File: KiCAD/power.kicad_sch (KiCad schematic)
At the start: 64 parts, among them IC10 ADP7182ACPZN-R7, IC11 NCP161ASN330T1G, IC4 NCP161ASN330T1G, IC5 NCP161ASN330T1G, IC6 NCP161ASN330T1G, IC7 NCP161ASN330T1G, IC8 LT1026CS8#PBF, IC9 ADP7118ARDZ

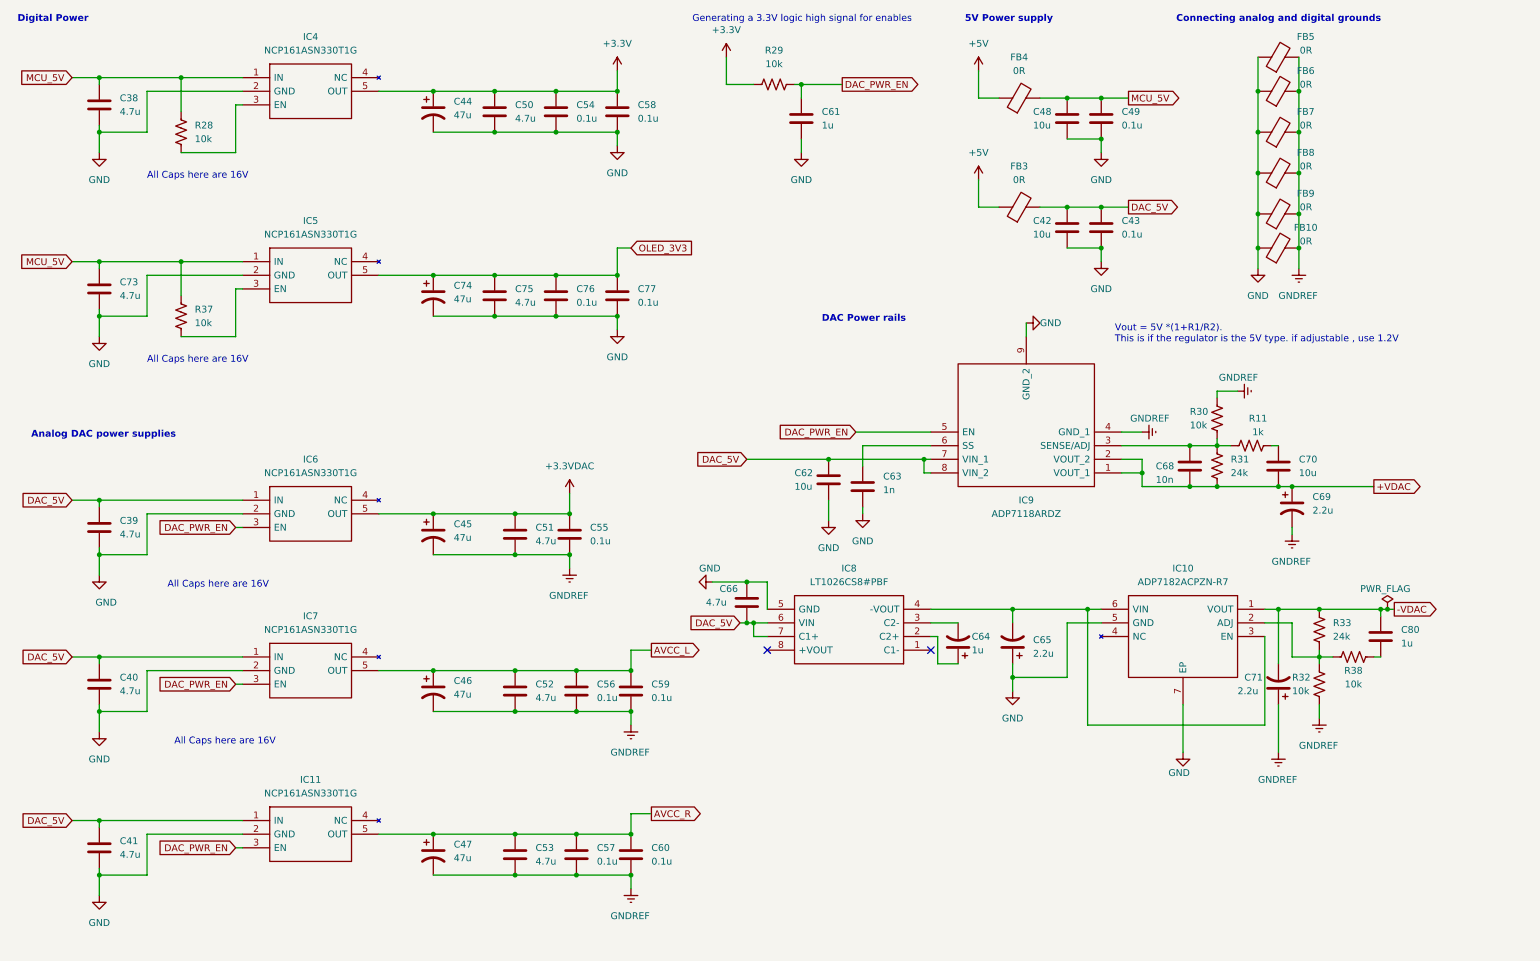
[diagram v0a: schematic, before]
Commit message: Adding stuff for rev 2.0
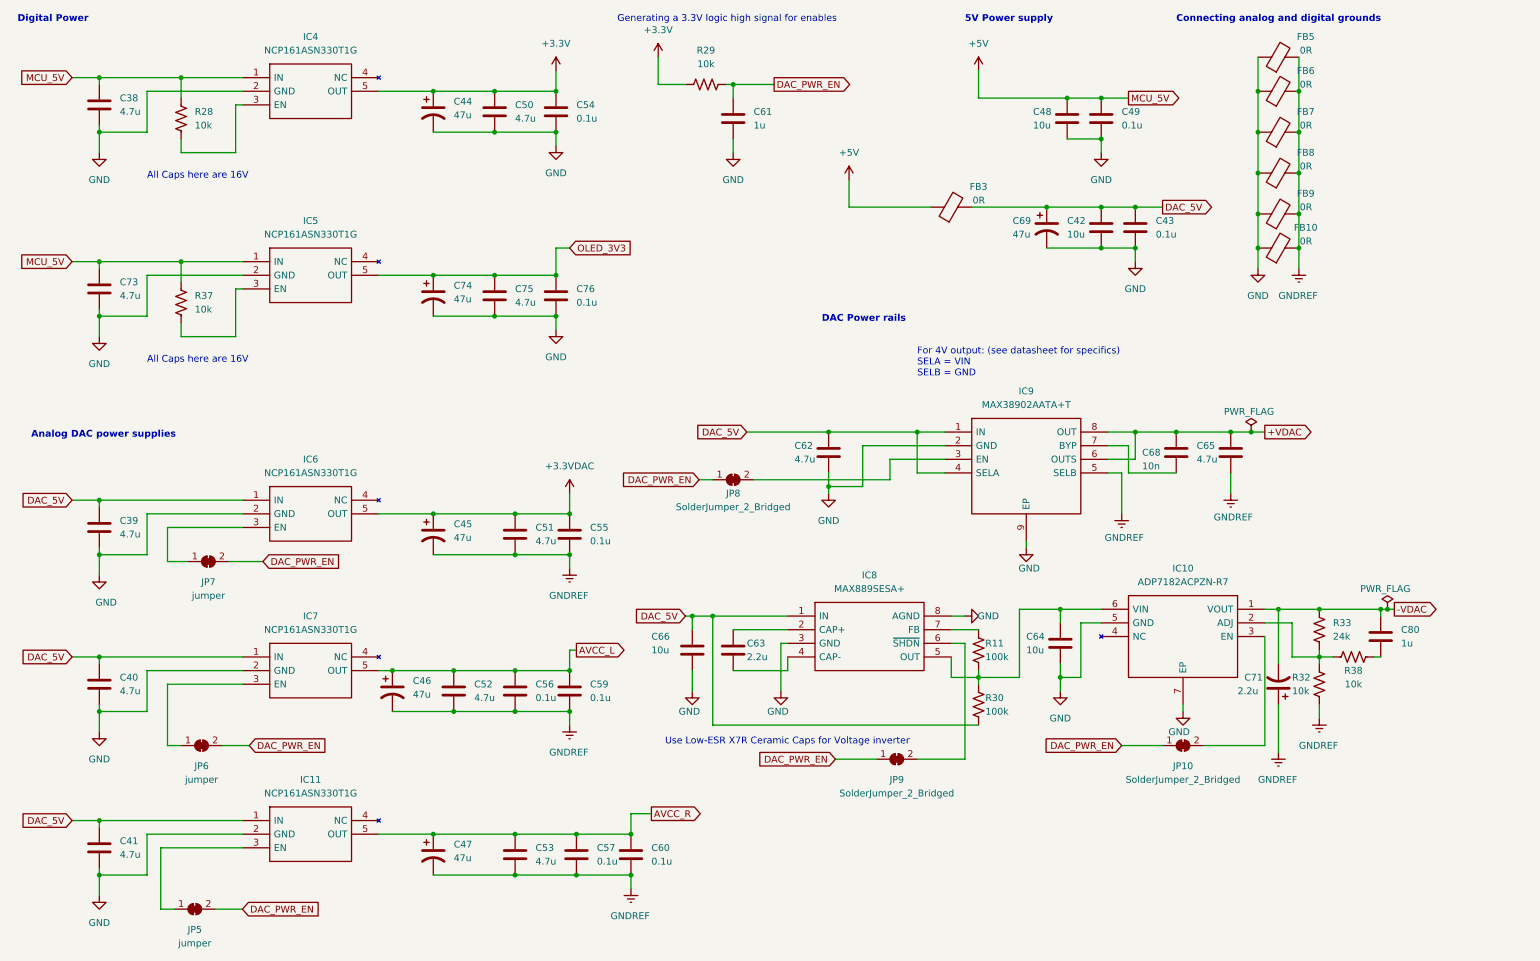
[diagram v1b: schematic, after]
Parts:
- removed C58, C77: 0.1u, Capacitor_SMD:C_0805_2012Metric_Pad1.18x1.45mm_HandSolder, symbol Device:C
- removed C64: 1u, Capacitor_THT:CP_Radial_D5.0mm_P2.00mm, symbol Device:C_Polarized_US
- removed C65: 2.2u, Capacitor_THT:CP_Radial_D4.0mm_P1.50mm, symbol Device:C_Polarized_US
- removed C70: 10u, Capacitor_SMD:C_0805_2012Metric_Pad1.18x1.45mm_HandSolder, symbol Device:C
- removed FB4: 0R, SamacSys_Parts:BEADC2012X110N, symbol Device:FerriteBead
- removed IC8: LT1026CS8#PBF, SamacSys_Parts:SOIC127P599X175-8N, symbol SamacSys_Parts:LT1026CS8#PBF
- removed IC9: ADP7118ARDZ, SOIC127P600X175-9N, symbol SamacSys_Parts:ADP7118ARDZ
- removed R31: 24k, Resistor_SMD:R_0805_2012Metric_Pad1.20x1.40mm_HandSolder, symbol Device:R_US
- added C64: 10u, Capacitor_SMD:C_0805_2012Metric_Pad1.18x1.45mm_HandSolder, symbol Device:C
- added C65: 4.7u, Capacitor_SMD:C_0805_2012Metric_Pad1.18x1.45mm_HandSolder, symbol Device:C
- added IC8: MAX889SESA+, SOIC127P600X175-8N, symbol SamacSys_Parts:MAX889SESA+
- added IC9: MAX38902AATA+T, SON50P200X200X80-9N-D, symbol SamacSys_Parts:MAX38902AATA+T
- added JP10, JP8, JP9: SolderJumper_2_Bridged, SolderJumper-2_P1.3mm_Bridged2Bar_Pad1.0x1.5mm, symbol Jumper:SolderJumper_2_Bridged
- added JP5, JP6, JP7: jumper, SolderJumper-2_P1.3mm_Bridged2Bar_Pad1.0x1.5mm, symbol Jumper:SolderJumper_2_Bridged
- C42, C48: Mouser Part Number 963-LMK212ABJ106KG8T -> 963-TMK212BBJ106KG-T; Part Number LMK212ABJ106KG8T -> TMK212BBJ106KG-T
- C62: value 10u -> 4.7u; Mouser Part Number 963-LMK212ABJ106KG8T -> 603-CC805KKX5R7BB475; Part Number LMK212ABJ106KG8T -> CC0805KKX5R7BB475
- C63: value 1n -> 2.2u; Mouser Part Number 581-0805YD102KAT2A -> 963-TMK212B7225KGHT; Part Number 0805YD102KAT2A -> TMK212B7225KGHT
- C66: value 4.7u -> 10u; Mouser Part Number 603-CC805KKX5R7BB475 -> 963-TMK212BBJ106KG-T; Part Number CC0805KKX5R7BB475 -> TMK212BBJ106KG-T
- C69: value 2.2u -> 47u; footprint Capacitor_THT:CP_Radial_D4.0mm_P1.50mm -> Capacitor_THT:CP_Radial_D5.0mm_P2.50mm; Mouser Part Number 667-ECE-A1HKA2R2 -> 667-ECA-1CHG470I; Part Number ECE-A1HKA2R2 -> ECA-1CHG470I
- R11: value 1k -> 100k; Mouser Part Number 667-ERA-6AEB102V -> 71-RCV0805100KJNEA; Part Number ERA-6AEB102V -> RCV0805100KJNEA
- R30: value 10k -> 100k; Mouser Part Number 603-RT0805BRD0710KL -> 71-RCV0805100KJNEA; Part Number RT0805BRD0710KL -> RCV0805100KJNEA
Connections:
- net MCU_5V is gone; now on net +5V: C38.1, C48.2, C49.1, C73.1, IC4.1 (IN), IC5.1 (IN), R28.2, R37.2
- net +VDAC: now also C68.1, C65.1, IC9.6 (OUTS), IC9.8 (OUT); no longer C68.2, C69.1
- net DAC_5V: now also C66.1, C69.1, R30.1, IC8.1 (IN), IC9.1 (IN), IC9.4 (SELA); no longer C66.2
- net DAC_PWR_EN: now also JP10.1 (A), JP5.2 (B), JP6.2 (B), JP7.2 (B), JP8.1 (A), JP9.1 (A); no longer IC11.3 (EN), IC6.3 (EN), IC7.3 (EN)
- net GND: now also C66.2, C69.2, C64.2, IC8.3 (GND), IC8.8 (AGND), IC9.2 (GND), IC9.9 (EP); no longer C63.2, C66.1
- net GNDREF: now also C65.2, IC9.5 (SELB); no longer C69.2, R30.2
- net at IC10.6 (VIN): now also R11.1, R30.2, C64.1, IC8.5 (OUT); no longer IC10.3 (EN)
- net at R11.2: now also IC8.7 (FB)
- net at C63.1: now also IC8.2 (CAP+)
- new net: IC6.3 (EN), JP7.1 (A)
- new net: C63.2, IC8.4 (CAP-)
- new net: IC8.6 (~{SHDN}), JP9.2 (B)
- new net: IC10.3 (EN), JP10.2 (B)
- new net: IC11.3 (EN), JP5.1 (A)
- new net: IC9.3 (EN), JP8.2 (B)
- new net: IC7.3 (EN), JP6.1 (A)
- new net: C68.2, IC9.7 (BYP)
- no-connect marks 2 -> 0
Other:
- note added: "For 4V output: (see datasheet for specifics) SELA = VIN SELB = GND"
- note added: "Use Low-ESR X7R Ceramic Caps for Voltage inverter"
- note removed: "Vout = 5V *(1+R1/R2). This is if the regulator is the 5V type. if adjustable , use 1.2V"
- moved on the sheet: C42, C43, C46, C52, C56, C59, C61, C62, C66, C68, R28, R29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
